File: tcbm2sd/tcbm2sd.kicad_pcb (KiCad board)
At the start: 2 copper layers, 56 x 91 mm, 13 parts, among them J2 JTAG, J3 debug, J4 AMS1117, J5 SD CARD, J7 debug, J8 C16-Exp-Port, U1 XC9572XL-VQ64, U2 Arduino_Pro_Mini

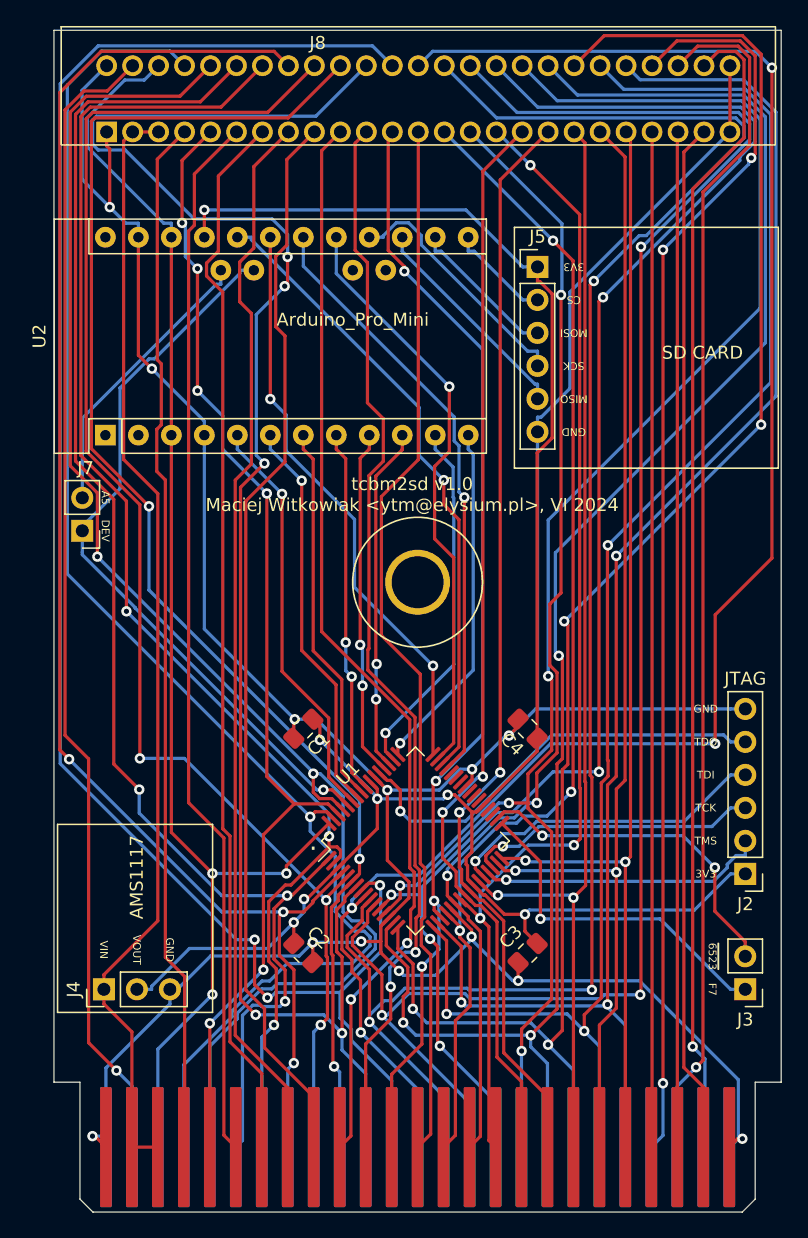
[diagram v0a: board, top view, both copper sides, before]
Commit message: clean pcb, new revision
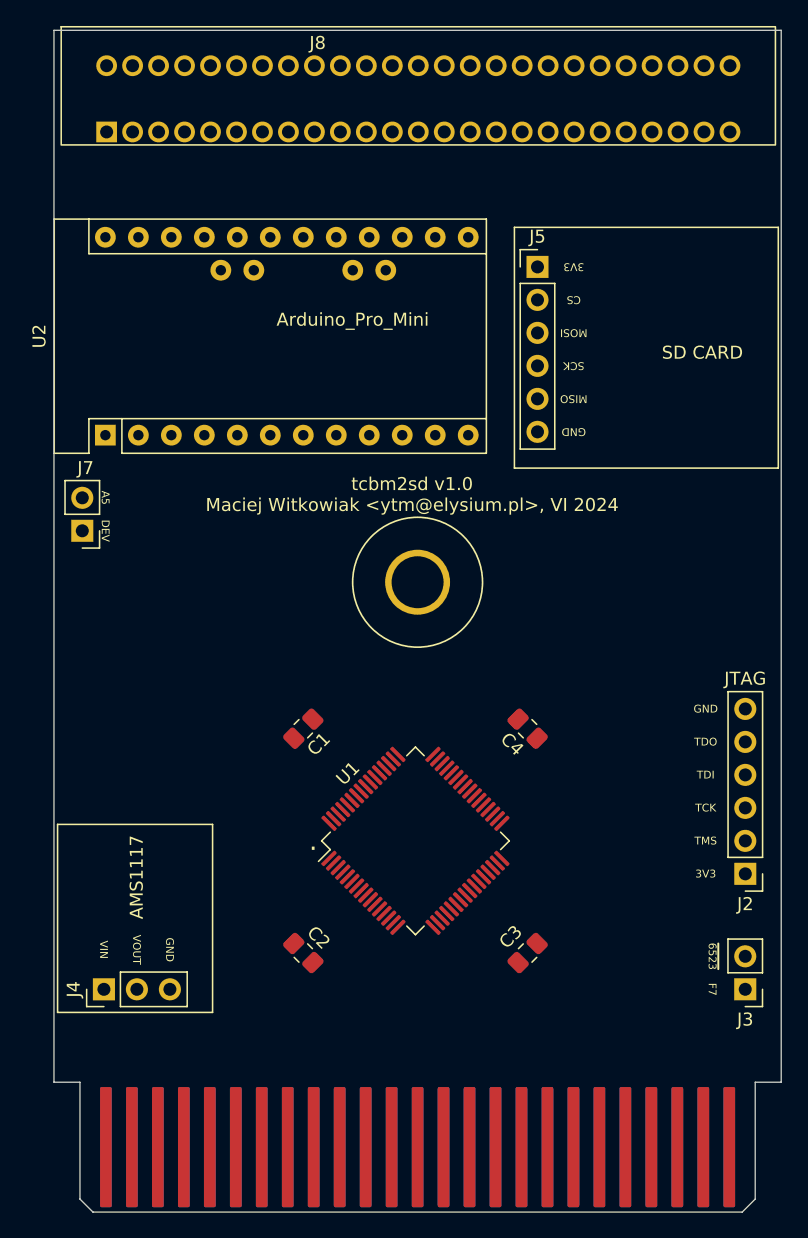
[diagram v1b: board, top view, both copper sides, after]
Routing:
- net GND: track 261.3 -> 0.00 mm, vias 13 -> 0
- net +3V3: track 152.7 -> 0.00 mm, vias 7 -> 0
- net /A8: track 138.3 -> 0.00 mm, vias 4 -> 0
- net /A7: track 138.2 -> 0.00 mm, vias 3 -> 0
- net /A6: track 138.0 -> 0.00 mm, vias 3 -> 0
- net /A9: track 135.9 -> 0.00 mm, vias 3 -> 0
- net /A10: track 134.1 -> 0.00 mm, vias 5 -> 0
- net /A2: track 126.5 -> 0.00 mm, vias 4 -> 0
- net /A3: track 125.1 -> 0.00 mm, vias 3 -> 0
- net /A4: track 123.7 -> 0.00 mm, vias 4 -> 0
- net /A5: track 120.3 -> 0.00 mm, vias 5 -> 0
- net /A1: track 118.9 -> 0.00 mm, vias 3 -> 0
- net /A13: track 117.2 -> 0.00 mm, vias 3 -> 0
- net /A0: track 116.9 -> 0.00 mm, vias 3 -> 0
- net /PHI0: track 115.3 -> 0.00 mm, vias 2 -> 0
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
